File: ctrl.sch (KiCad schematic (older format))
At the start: 56 parts, among them J1 OSC-I, J10 LCDD/DAH, J11 ROT/S, J12 GND, J13 BAND/SIDE, J14 GND, J15 TX/KEY, J16 OSC-TX, J17 Supply, J18 PTT, J19 Conn_01x01, J2 OSC-Q, J20 Conn_01x01, J3 Supply, J4 SI5351, J5 Dit, J6 TX/KEY, J7 GND, J8 DSupply, J9 DCtrl, Q1 2N3904, U1 74HC74, U2 ATmega328-PU, U3 L7805, Y1 20MHz

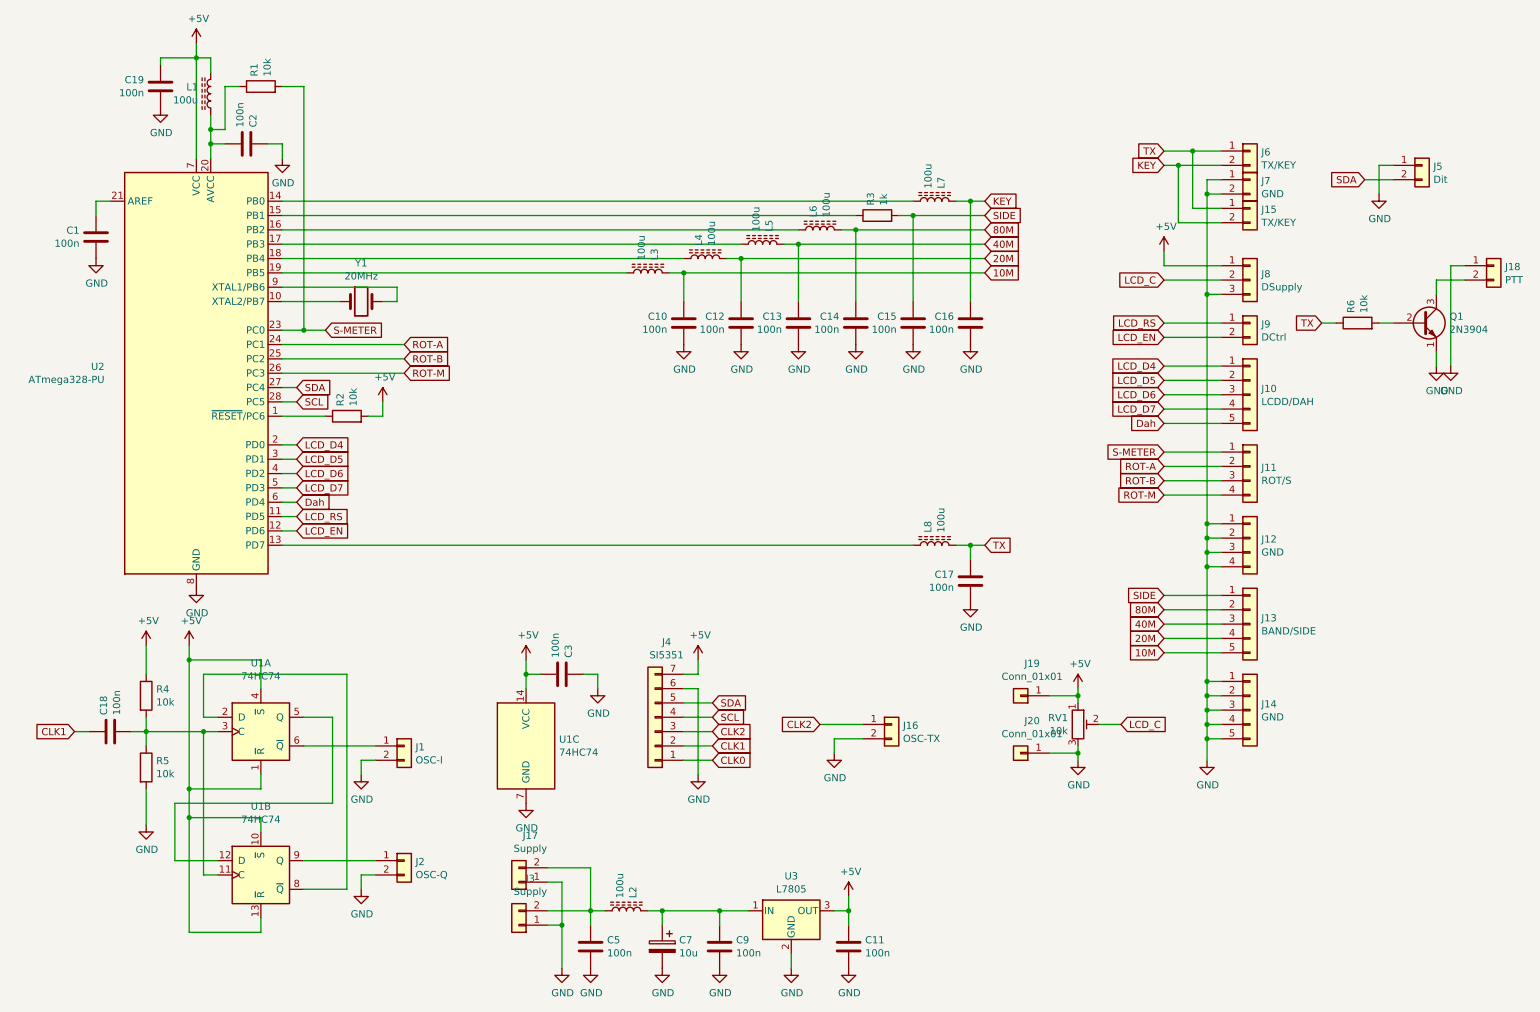
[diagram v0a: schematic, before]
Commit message: Fixed minors.
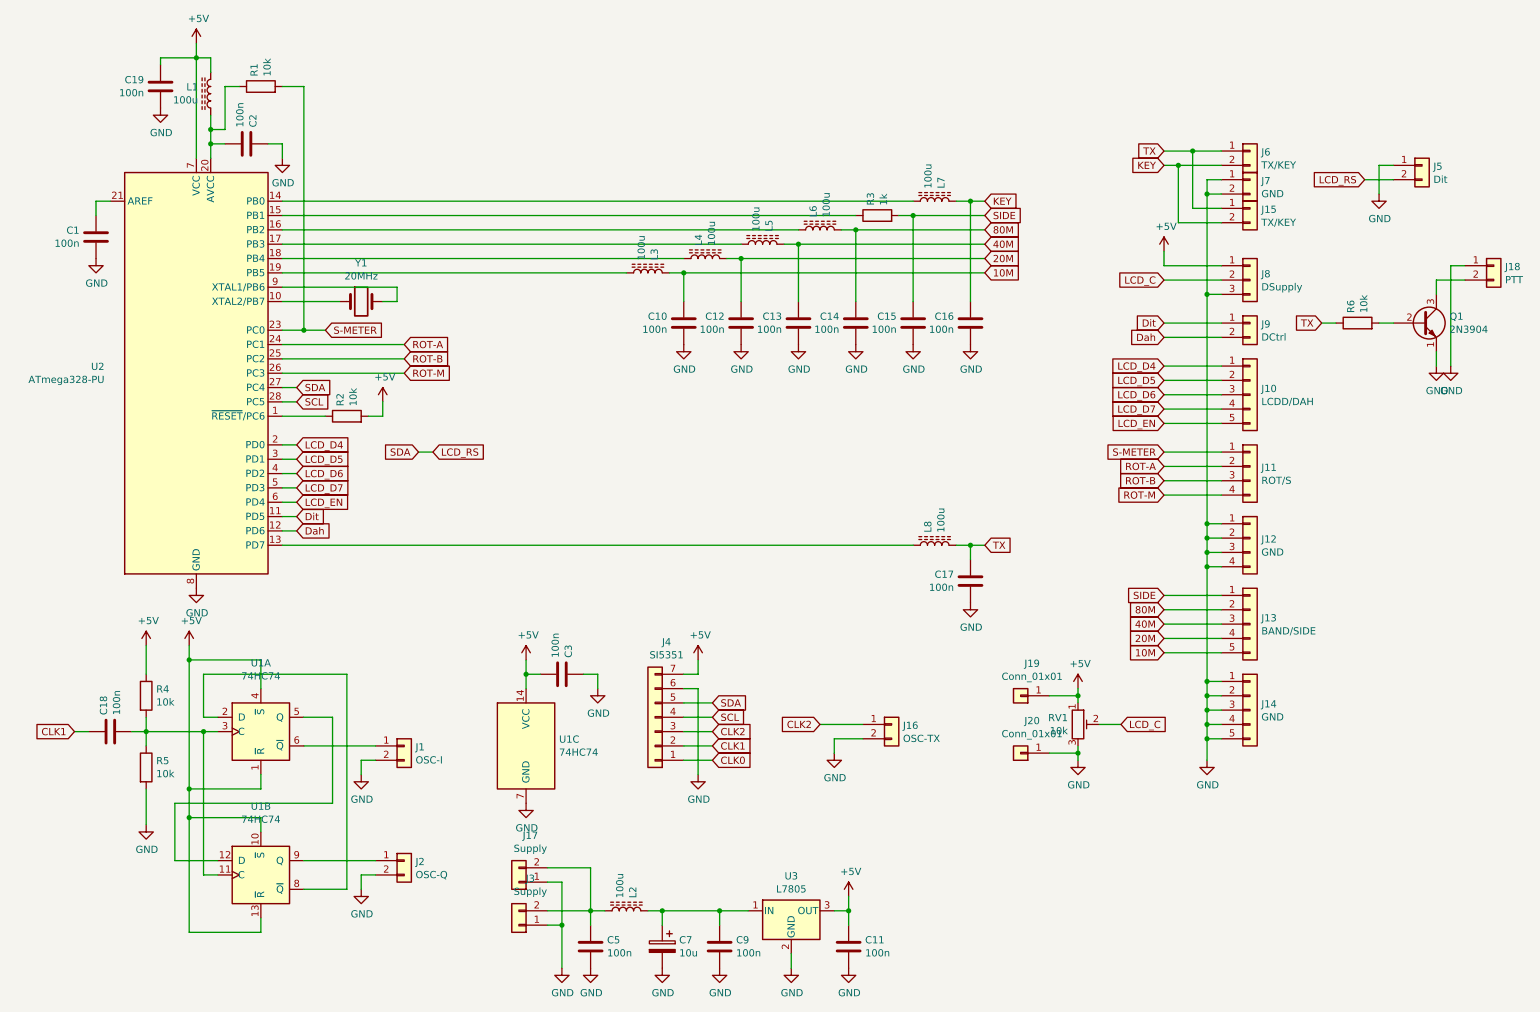
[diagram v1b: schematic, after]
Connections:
- net SDA is gone; now on net LCD_RS: J4.5 (Pin_5), J5.2 (Pin_2), U2.27 (PC4)
- net Dah: now also J9.2 (Pin_2), U2.12 (PD6); no longer J10.5 (Pin_5), U2.6 (PD4)
- net LCD_EN: now also J10.5 (Pin_5), U2.6 (PD4); no longer J9.2 (Pin_2), U2.12 (PD6)
- net LCD_RS: no longer J9.1 (Pin_1), U2.11 (PD5)
- new net Dit: J9.1 (Pin_1), U2.11 (PD5)
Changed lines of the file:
@@
 Text GLabel 2550 3950 2    50   Input ~ 0
 LCD_D7
-Text GLabel 2550 4150 2    50   Input ~ 0
+Text GLabel 3500 3700 2    50   Input ~ 0
 LCD_RS
-Text GLabel 2550 4250 2    50   Input ~ 0
+Text GLabel 2550 4050 2    50   Input ~ 0
 LCD_EN
 Wire Wire Line
@@
 Connection ~ 7250 1950
 Wire Wire Line
-	2450 4250 2550 4250
-Wire Wire Line
-	2550 4150 2450 4150
-Wire Wire Line
 	7250 4350 7350 4350
 Wire Wire Line
@@
 Wire Wire Line
 	8600 2500 9000 2500
-Text GLabel 8600 2800 0    50   Input ~ 0
+Text GLabel 10000 1800 0    50   Input ~ 0
 LCD_RS
-Text GLabel 8600 2900 0    50   Input ~ 0
+Text GLabel 8600 3500 0    50   Input ~ 0
 LCD_EN
-Wire Wire Line
-	8600 2800 9000 2800
-Wire Wire Line
-	8600 2900 9000 2900
 Text GLabel 8600 3100 0    50   Input ~ 0
 LCD_D4
@@
 Wire Wire Line
 	10100 1700 10100 1900
-Text GLabel 10000 1800 0    50   Input ~ 0
-SDA
-Wire Wire Line
-	10000 1800 10200 1800
 $Comp
 L Connector_Generic:Conn_01x02 J5
@@
 	1    0    0    -1
 $EndComp
-Text GLabel 8600 3500 0    50   Input ~ 0
+Text GLabel 8600 2900 0    50   Input ~ 0
 Dah
-Wire Wire Line
-	8600 3500 9000 3500
-Text GLabel 2550 4050 2    50   Input ~ 0
+Text GLabel 2550 4250 2    50   Input ~ 0
 Dah
-Wire Wire Line
-	2450 4050 2550 4050
 $Comp
 L Device:R R4
@@
 Wire Wire Line
 	2450 2950 3300 2950
+Wire Wire Line
+	8600 3500 9000 3500
+Wire Wire Line
+	2550 4050 2450 4050
+Text GLabel 2550 4150 2    50   Input ~ 0
+Dit
+Wire Wire Line
+	2550 4150 2450 4150
+Wire Wire Line
+	2450 4250 2550 4250
+Text GLabel 3400 3700 0    50   Input ~ 0
+SDA
+Wire Wire Line
+	3400 3700 3500 3700
+Wire Wire Line
+	10000 1800 10200 1800
+Text GLabel 8600 2800 0    50   Input ~ 0
+Dit
+Wire Wire Line
+	8600 2800 9000 2800
+Wire Wire Line
+	8600 2900 9000 2900
 $EndSCHEMATC
